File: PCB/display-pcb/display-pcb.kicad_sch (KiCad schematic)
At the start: 9 parts, among them J1 B6B-XH-A, J2 B8B-XH-A, SW1 PTS645SL50-2 LFS, SW2 PTS645SL50-2 LFS, SW3 PTS645SL50-2 LFS, SW4 PTS645SL50-2 LFS, U1 NHD-C12864A1Z

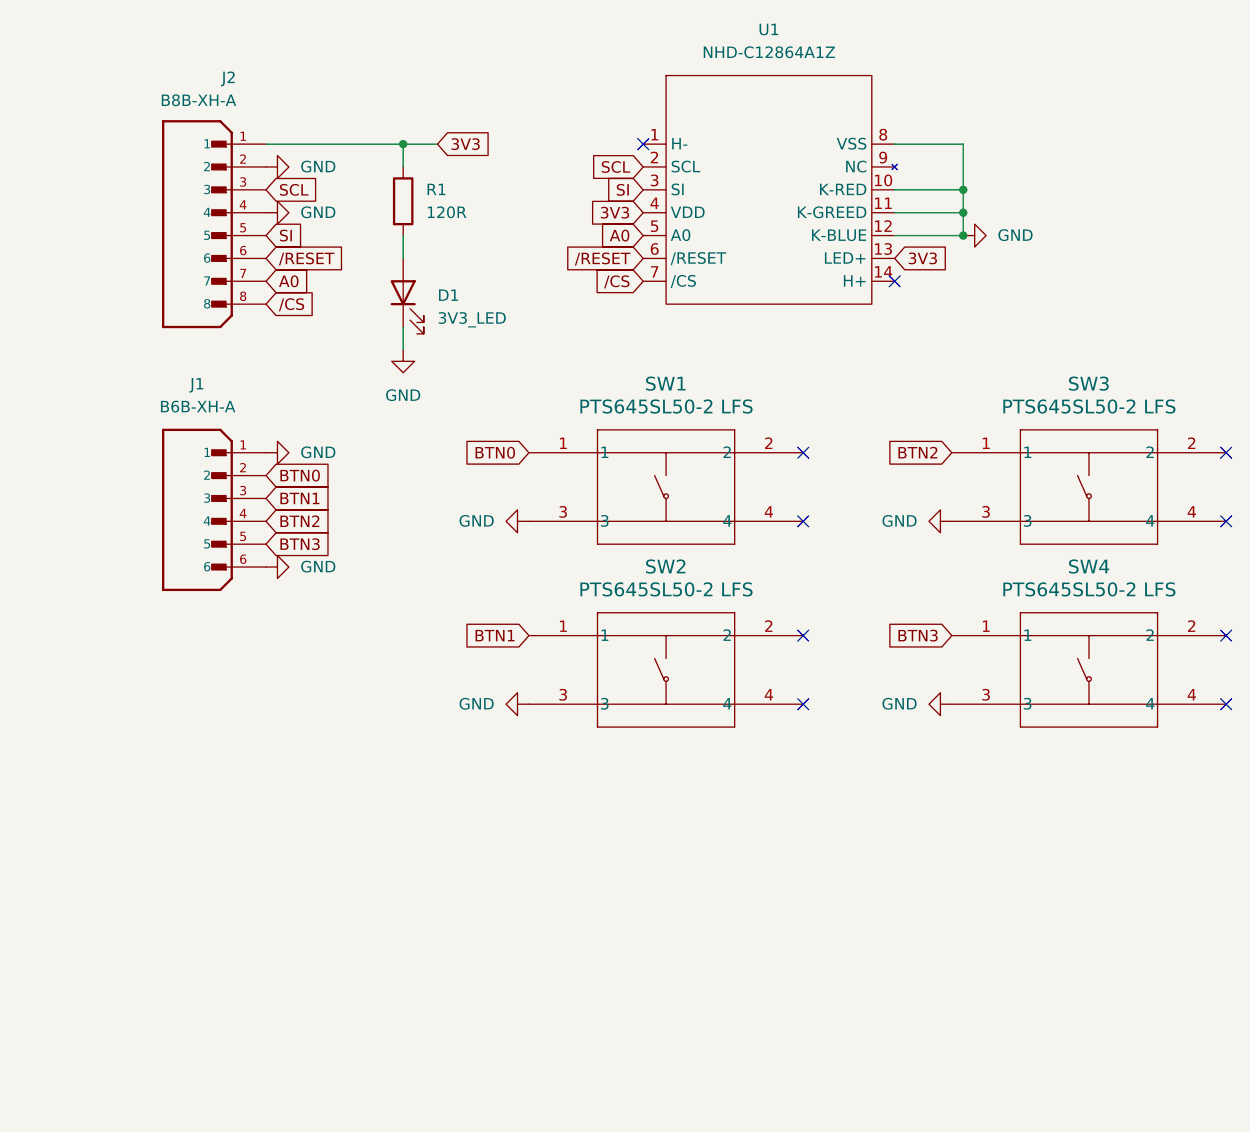
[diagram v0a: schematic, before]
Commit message: PCB updates
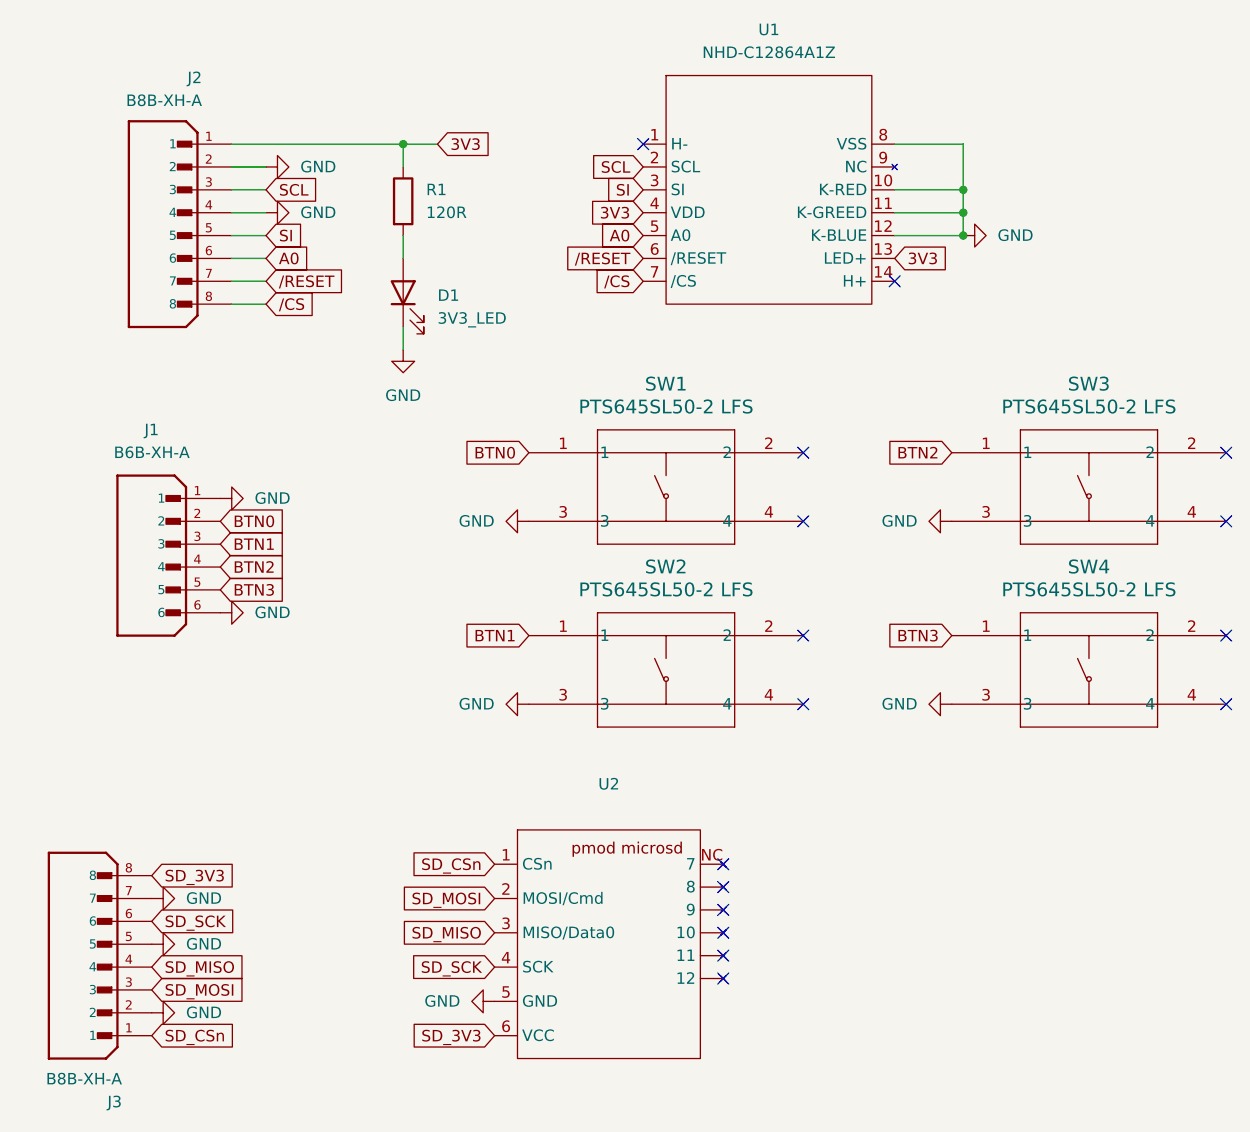
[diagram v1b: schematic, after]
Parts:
- added J3: B8B-XH-A, Connector_JST:JST_XH_B8B-XH-A_1x08_P2.50mm_Vertical, symbol B8B-XH-A:B8B-XH-A
- added U2: ~, microsd:pmod-microsd, symbol microsd-2:pmod-microsd
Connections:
- net A0: now also J2.6; no longer J2.7
- net GND: now also J3.2, J3.5, J3.7, U2.5 (GND)
- net /RESET: now also J2.7; no longer J2.6
- new net SD_3V3: J3.8, U2.6 (VCC)
- new net SD_CSn: J3.1, U2.1 (CSn)
- new net SD_MISO: J3.4, U2.3 (MISO/Data0)
- new net SD_MOSI: J3.3, U2.2 (MOSI/Cmd)
- new net SD_SCK: J3.6, U2.4 (SCK)
- no-connect marks 10 -> 16
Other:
- moved on the sheet: J1, J2

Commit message: pcb finishing touches
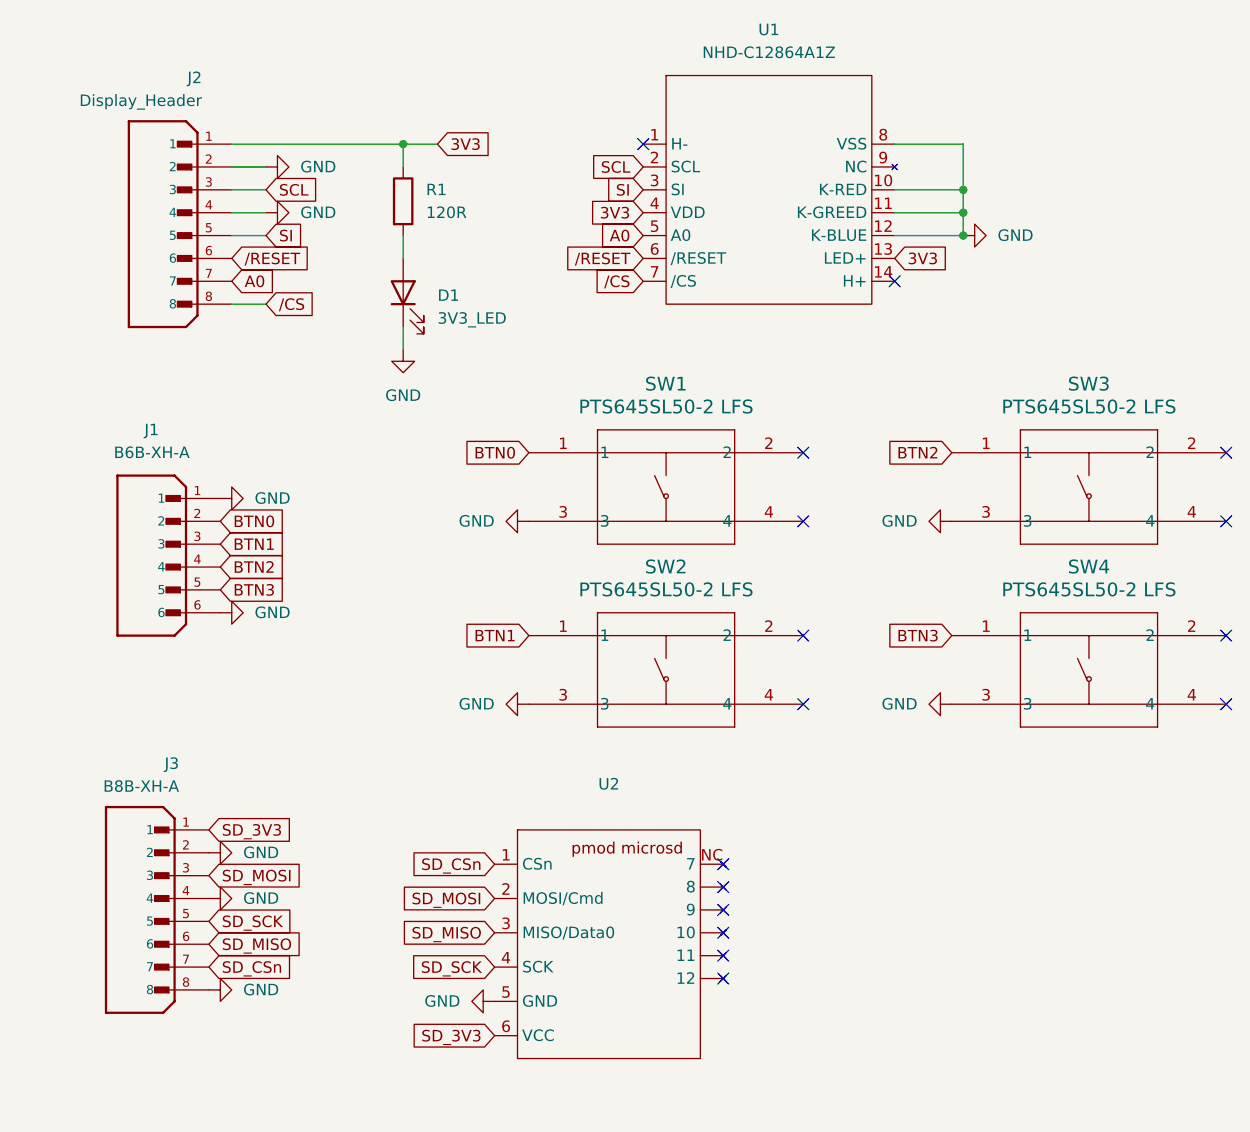
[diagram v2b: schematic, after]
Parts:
- J2: value B8B-XH-A -> Display_Header
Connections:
- net A0: now also J2.7; no longer J2.6
- net GND: now also J3.4, J3.8; no longer J3.5, J3.7
- net SD_3V3: now also J3.1; no longer J3.8
- net SD_CSn: now also J3.7; no longer J3.1
- net SD_MISO: now also J3.6; no longer J3.4
- net SD_SCK: now also J3.5; no longer J3.6
- net /RESET: now also J2.6; no longer J2.7
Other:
- moved on the sheet: J3
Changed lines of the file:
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@@
 	(wire
 		(pts
-			(xy 86.36 71.12) (xy 90.17 71.12)
+			(xy 160.02 60.96) (xy 167.64 60.96)
 		)
 		(stroke
@@
 	(wire
 		(pts
-			(xy 86.36 68.58) (xy 90.17 68.58)
+			(xy 105.41 55.88) (xy 105.41 58.42)
 		)
 		(stroke
@@
 	(wire
 		(pts
-			(xy 160.02 60.96) (xy 167.64 60.96)
+			(xy 86.36 55.88) (xy 105.41 55.88)
 		)
 		(stroke
@@
 	(wire
 		(pts
-			(xy 105.41 55.88) (xy 105.41 58.42)
+			(xy 86.36 60.96) (xy 90.17 60.96)
 		)
 		(stroke
@@
 	(wire
 		(pts
-			(xy 86.36 55.88) (xy 105.41 55.88)
+			(xy 167.64 55.88) (xy 167.64 60.96)
 		)
 		(stroke
@@
 	(wire
 		(pts
-			(xy 86.36 60.96) (xy 90.17 60.96)
+			(xy 160.02 55.88) (xy 167.64 55.88)
 		)
 		(stroke
@@
 	(wire
 		(pts
-			(xy 167.64 55.88) (xy 167.64 60.96)
+			(xy 86.36 73.66) (xy 90.17 73.66)
 		)
 		(stroke
@@
 	(wire
 		(pts
-			(xy 160.02 55.88) (xy 167.64 55.88)
+			(xy 167.64 63.5) (xy 167.64 66.04)
 		)
 		(stroke
@@
 	(wire
 		(pts
-			(xy 86.36 73.66) (xy 90.17 73.66)
+			(xy 86.36 66.04) (xy 90.17 66.04)
 		)
 		(stroke
@@
 	(wire
 		(pts
-			(xy 167.64 63.5) (xy 167.64 66.04)
+			(xy 105.41 78.74) (xy 105.41 76.2)
 		)
 		(stroke
@@
 	(wire
 		(pts
-			(xy 86.36 66.04) (xy 90.17 66.04)
+			(xy 86.36 63.5) (xy 90.17 63.5)
 		)
 		(stroke
@@
 	(wire
 		(pts
-			(xy 105.41 78.74) (xy 105.41 76.2)
+			(xy 160.02 66.04) (xy 167.64 66.04)
 		)
 		(stroke
@@
 	(wire
 		(pts
-			(xy 86.36 63.5) (xy 90.17 63.5)
+			(xy 167.64 60.96) (xy 167.64 63.5)
 		)
 		(stroke
@@
 	(wire
 		(pts
-			(xy 160.02 66.04) (xy 167.64 66.04)
+			(xy 105.41 55.88) (xy 109.22 55.88)
 		)
 		(stroke
@@
 		)
 	)
-	(wire
-		(pts
-			(xy 167.64 60.96) (xy 167.64 63.5)
-		)
-		(stroke
-			(width 0)
-			(type default)
-		)
-	)
-	(wire
-		(pts
-			(xy 105.41 55.88) (xy 109.22 55.88)
-		)
-		(stroke
-			(width 0)
-			(type default)
-		)
-	)
 	(global_label "A0"
 		(shape input)
-		(at 90.17 68.58 0)
+		(at 86.36 71.12 0)
 		(fields_autoplaced yes)
 		(effects
@@
 		)
 		(property "Intersheetrefs" "${INTERSHEET_REFS}"
-			(at 95.4533 68.58 0)
+			(at 91.6433 71.12 0)
 			(effects
 				(font
@@
 	(global_label "SD_MISO"
 		(shape input)
-		(at 77.47 147.32 0)
+		(at 83.82 144.78 0)
 		(fields_autoplaced yes)
 		(effects
@@
 		)
 		(property "Intersheetrefs" "${INTERSHEET_REFS}"
-			(at 88.4985 147.32 0)
+			(at 94.8485 144.78 0)
 			(effects
 				(font
@@
 	(global_label "SD_MOSI"
 		(shape input)
-		(at 77.47 149.86 0)
+		(at 83.82 137.16 0)
 		(fields_autoplaced yes)
 		(effects
@@
 		)
 		(property "Intersheetrefs" "${INTERSHEET_REFS}"
-			(at 88.4985 149.86 0)
+			(at 94.8485 137.16 0)
 			(effects
 				(font
@@
 	(global_label "SD_SCK"
 		(shape input)
-		(at 77.47 142.24 0)
+		(at 83.82 142.24 0)
 		(fields_autoplaced yes)
 		(effects
@@
 		)
 		(property "Intersheetrefs" "${INTERSHEET_REFS}"
-			(at 87.6518 142.24 0)
+			(at 94.0018 142.24 0)
 			(effects
 				(font
@@
 	(global_label "{slash}RESET"
 		(shape input)
-		(at 90.17 71.12 0)
+		(at 86.36 68.58 0)
 		(fields_autoplaced yes)
 		(effects
@@
 		)
 		(property "Intersheetrefs" "${INTERSHEET_REFS}"
-			(at 100.2308 71.12 0)
+			(at 96.4208 68.58 0)
 			(effects
 				(font
@@
 	(global_label "SD_CSn"
 		(shape input)
-		(at 77.47 154.94 0)
+		(at 83.82 147.32 0)
 		(fields_autoplaced yes)
 		(effects
@@
 		)
 		(property "Intersheetrefs" "${INTERSHEET_REFS}"
-			(at 87.5308 154.94 0)
+			(at 93.8808 147.32 0)
 			(effects
 				(font
@@
 	(global_label "SD_3V3"
 		(shape input)
-		(at 77.47 137.16 0)
+		(at 83.82 132.08 0)
 		(fields_autoplaced yes)
 		(effects
@@
 		)
 		(property "Intersheetrefs" "${INTERSHEET_REFS}"
-			(at 87.4099 137.16 0)
+			(at 93.7599 132.08 0)
 			(effects
 				(font
@@
 			)
 		)
-		(property "Value" "B8B-XH-A"
+		(property "Value" "Display_Header"
 			(at 83.058 51.054 0)
 			(effects
@@
 	(symbol
 		(lib_id "B8B-XH-A:B8B-XH-A")
-		(at 69.85 144.78 180)
+		(at 76.2 142.24 0)
+		(mirror y)
 		(unit 1)
 		(exclude_from_sim no)
@@
 		(dnp no)
 		(property "Reference" "J3"
-			(at 74.168 162.306 0)
+			(at 80.518 124.714 0)
 			(effects
 				(font
@@
 		)
 		(property "Value" "B8B-XH-A"
-			(at 74.168 159.766 0)
+			(at 80.518 127.254 0)
 			(effects
 				(font
@@
 		)
 		(property "Footprint" "Connector_JST:JST_XH_B8B-XH-A_1x08_P2.50mm_Vertical"
-			(at 69.85 144.78 0)
+			(at 76.2 142.24 0)
 			(effects
 				(font
@@
 		)
 		(property "Datasheet" ""
-			(at 69.85 144.78 0)
+			(at 76.2 142.24 0)
 			(effects
 				(font
@@
 		)
 		(property "Description" ""
-			(at 69.85 144.78 0)
+			(at 76.2 142.24 0)
 			(effects
 				(font
@@
 		)
 		(property "PARTREV" "7/4/21"
-			(at 69.85 144.78 0)
+			(at 76.2 142.24 0)
 			(effects
 				(font
@@
 		)
 		(property "STANDARD" "Manufacturer Recommendations"
-			(at 69.85 144.78 0)
+			(at 76.2 142.24 0)
 			(effects
 				(font
@@
 		)
 		(property "MAXIMUM_PACKAGE_HEIGHT" "7.00 mm"
-			(at 69.85 144.78 0)
+			(at 76.2 142.24 0)
 			(effects
 				(font
@@
 		)
 		(property "MANUFACTURER" "JST"
-			(at 69.85 144.78 0)
+			(at 76.2 142.24 0)
 			(effects
 				(font
@@
 	(symbol
 		(lib_id "power:GND")
-		(at 77.47 152.4 90)
+		(at 83.82 149.86 90)
 		(unit 1)
 		(exclude_from_sim no)
@@
 		(fields_autoplaced yes)
 		(property "Reference" "#PWR013"
-			(at 83.82 152.4 0)
+			(at 90.17 149.86 0)
 			(effects
 				(font
@@
 		)
 		(property "Value" "GND"
-			(at 81.28 152.3999 90)
+			(at 87.63 149.8599 90)
 			(effects
 				(font
@@
 		)
 		(property "Footprint" ""
-			(at 77.47 152.4 0)
+			(at 83.82 149.86 0)
 			(effects
 				(font
@@
 		)
 		(property "Datasheet" ""
-			(at 77.47 152.4 0)
+			(at 83.82 149.86 0)
 			(effects
 				(font
@@
 		)
 		(property "Description" "Power symbol creates a global label with name \"GND\" , ground"
-			(at 77.47 152.4 0)
+			(at 83.82 149.86 0)
 			(effects
 				(font
@@
 	(symbol
 		(lib_id "power:GND")
-		(at 77.47 139.7 90)
+		(at 83.82 134.62 90)
 		(unit 1)
 		(exclude_from_sim no)
@@
 		(fields_autoplaced yes)
 		(property "Reference" "#PWR014"
-			(at 83.82 139.7 0)
+			(at 90.17 134.62 0)
 			(effects
 				(font
@@
 		)
 		(property "Value" "GND"
-			(at 81.28 139.6999 90)
+			(at 87.63 134.6199 90)
 			(effects
 				(font
@@
 		)
 		(property "Footprint" ""
-			(at 77.47 139.7 0)
+			(at 83.82 134.62 0)
 			(effects
 				(font
@@
 		)
 		(property "Datasheet" ""
-			(at 77.47 139.7 0)
+			(at 83.82 134.62 0)
 			(effects
 				(font
@@
 		)
 		(property "Description" "Power symbol creates a global label with name \"GND\" , ground"
-			(at 77.47 139.7 0)
+			(at 83.82 134.62 0)
 			(effects
 				(font
@@
 	(symbol
 		(lib_id "power:GND")
-		(at 77.47 144.78 90)
+		(at 83.82 139.7 90)
 		(unit 1)
 		(exclude_from_sim no)
@@
 		(fields_autoplaced yes)
 		(property "Reference" "#PWR011"
-			(at 83.82 144.78 0)
+			(at 90.17 139.7 0)
 			(effects
 				(font
@@
 		)
 		(property "Value" "GND"
-			(at 81.28 144.7799 90)
+			(at 87.63 139.6999 90)
 			(effects
 				(font
@@
 		)
 		(property "Footprint" ""
-			(at 77.47 144.78 0)
+			(at 83.82 139.7 0)
 			(effects
 				(font
@@
 		)
 		(property "Datasheet" ""
-			(at 77.47 144.78 0)
+			(at 83.82 139.7 0)
 			(effects
 				(font
@@
 		)
 		(property "Description" "Power symbol creates a global label with name \"GND\" , ground"
-			(at 77.47 144.78 0)
-			(effects
-				(font
+			(at 83.82 139.7 0)
+			(effects
+				(font

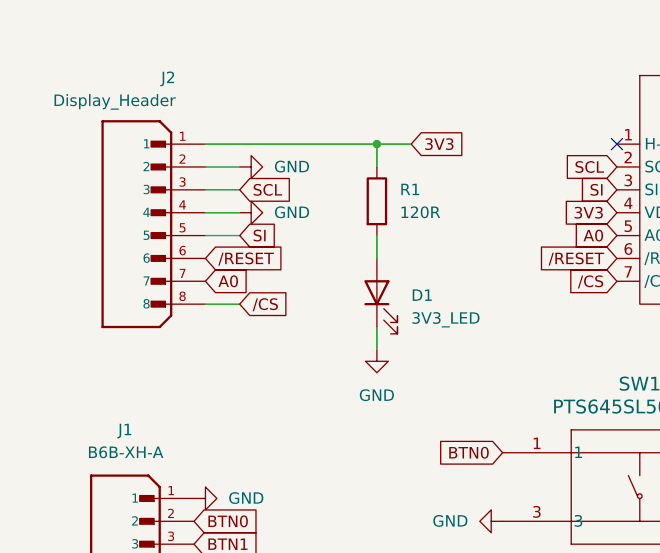
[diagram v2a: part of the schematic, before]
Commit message: gerbs
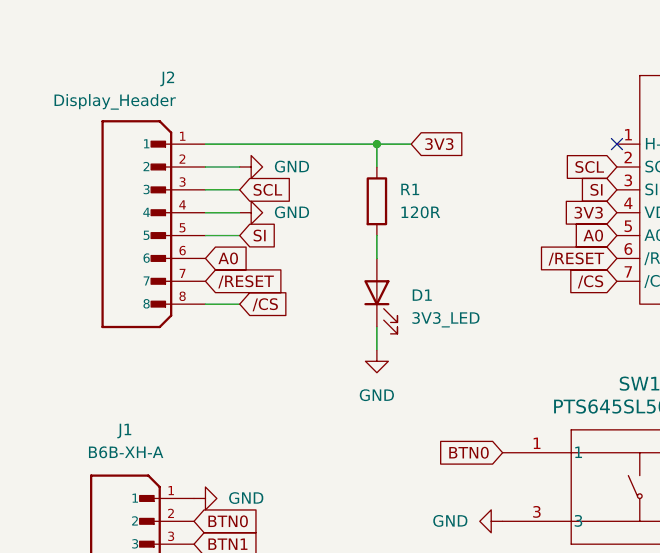
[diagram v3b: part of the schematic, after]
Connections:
- net A0: now also J2.6; no longer J2.7
- net /RESET: now also J2.7; no longer J2.6
